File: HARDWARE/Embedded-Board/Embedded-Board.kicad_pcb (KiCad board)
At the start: 2 copper layers, 80 x 60 mm, 81 parts, among them J1 AD7265X, J11 USB_C_Receptacle_USB2.0, J2 POWER-pins, J3 Conn_02x20_Odd_Even, J4 AD7341, J5 I2C comm, J6 GPIO PINS, Q1 MMUN2133LT1G, SW1 SW_Push, SW2 RotaryEncoder_Switch, SW3 SW_Push_SPDT, SW5 BOOT, U1 MCP73831-2-OT, U18 LM1117-3.3, U2 W25Q16JVS, U3 RP2040, U4 TPS61090, Y1 12MHz

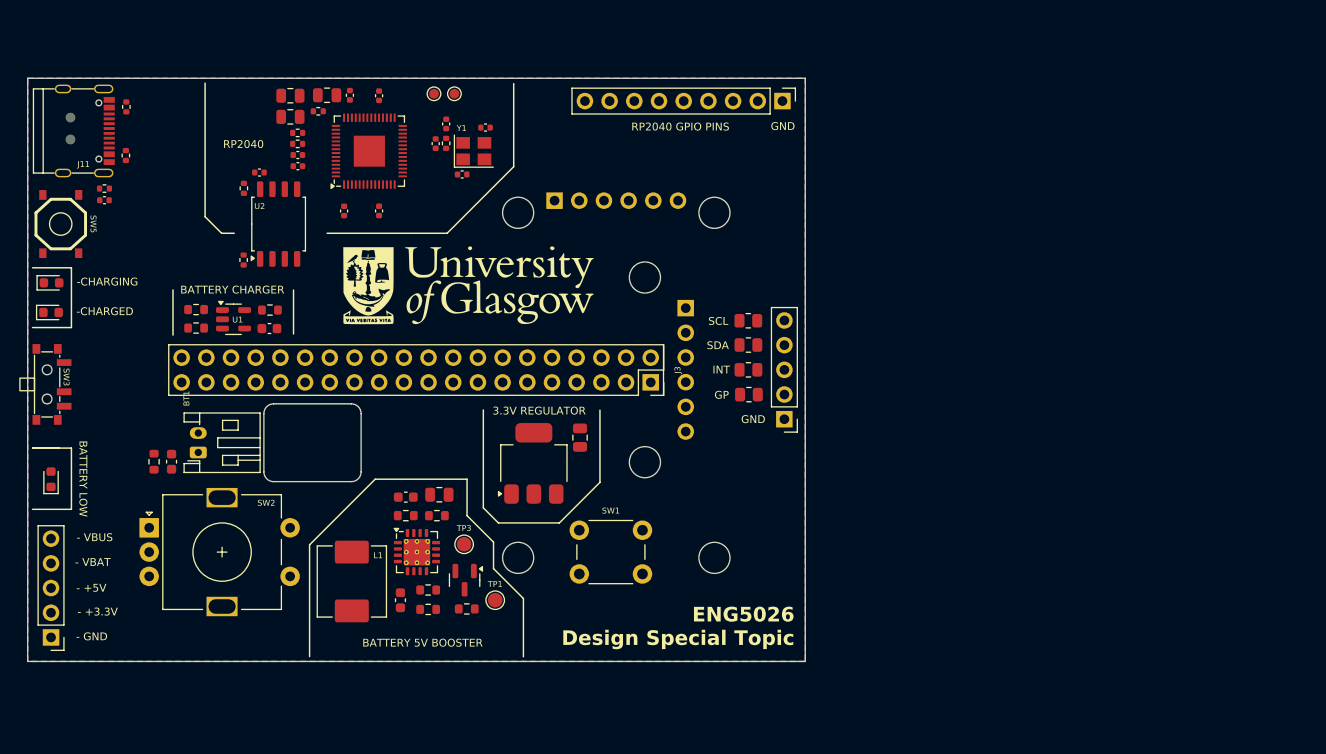
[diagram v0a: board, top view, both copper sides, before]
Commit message: Final PCB version
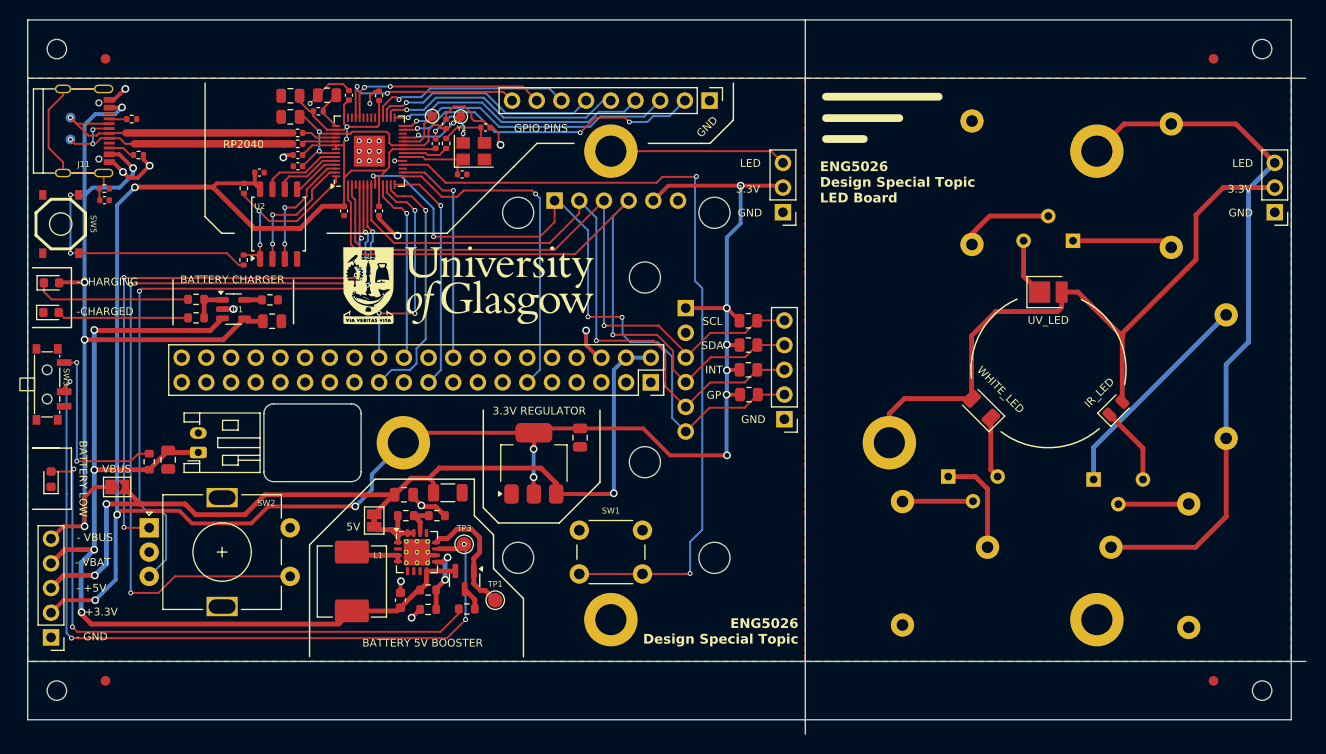
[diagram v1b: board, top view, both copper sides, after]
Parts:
- added D4: WHITE-LED, LED_SMD:LED_1206_3216Metric, F.Cu at (173.2, 88.6)
- added D5: IR_LED, LED_SMD:LED_0805_2012Metric, F.Cu at (187.1, 88.6)
- added D6: UV_LED, LED_SMD:LED_PLCC_2835, F.Cu at (180.2, 76.7)
- added G***: LOGO, test:uofg-8mm, B.Cu at (180.2, 84.7)
- added J7: BOARD->LED, Connector_PinHeader_2.54mm:PinHeader_1x03_P2.54mm_Vertical, F.Cu at (152.8, 68.4)
- added J8: LED->BOARD, Connector_PinHeader_2.54mm:PinHeader_1x03_P2.54mm_Vertical, F.Cu at (203.4, 68.4)
- added JP1: VBUS-5V, Jumper:SolderJumper-2_P1.3mm_Open_TrianglePad1.0x1.5mm, F.Cu at (84.3, 96.7)
- added JP2: OUT-5V, Jumper:SolderJumper-2_P1.3mm_Bridged_Pad1.0x1.5mm, F.Cu at (110.8, 100.2)
- added Q3: Q_NPN_BEC, Package_TO_SOT_THT:TO-92_Wide, B.Cu at (169.9, 95.6)
- added Q4: Q_NPN_BEC, Package_TO_SOT_THT:TO-92_Wide, B.Cu at (184.8, 95.9)
- added Q5: Q_NPN_BEC, Package_TO_SOT_THT:TO-92_Wide, B.Cu at (182.7, 71.4)
- added R23: 10k, Resistor_THT:R_Axial_DIN0411_L9.9mm_D3.6mm_P12.70mm_Horizontal, B.Cu at (186.6, 102.9)
- added R24: 10k, Resistor_THT:R_Axial_DIN0411_L9.9mm_D3.6mm_P12.70mm_Horizontal, B.Cu at (198.4, 91.7)
- added R25: 10k, Resistor_THT:R_Axial_DIN0411_L9.9mm_D3.6mm_P12.70mm_Horizontal, B.Cu at (192.8, 59.4)
- added R26: 470, Resistor_THT:R_Axial_DIN0411_L9.9mm_D3.6mm_P12.70mm_Horizontal, B.Cu at (165.2, 110.9)
- added R27: 470, Resistor_THT:R_Axial_DIN0411_L9.9mm_D3.6mm_P12.70mm_Horizontal, B.Cu at (194.6, 111.2)
- added R28: 470, Resistor_THT:R_Axial_DIN0411_L9.9mm_D3.6mm_P12.70mm_Horizontal, B.Cu at (172.3, 59.0)
- added REF**: Fiducial_1mm_Mask3mm, Fiducial:Fiducial_1mm_Mask3mm, F.Cu at (197.1, 116.6)
- added REF**: TestPoint, user:1.3mm_Test_Point, F.Cu at (202.2, 51.6)
- added REF**: Fiducial_1mm_Mask3mm, Fiducial:Fiducial_1mm_Mask3mm, F.Cu at (83.2, 52.7)
- added REF**: MountingHole_3.2mm_M3_ISO14580_Pad, MountingHole:MountingHole_3.2mm_M3_ISO14580_Pad, F.Cu at (185.2, 62.1)
- added REF**: TestPoint, user:1.3mm_Test_Point, F.Cu at (202.1, 117.7)
- added REF**: MountingHole_3.2mm_M3_ISO14580_Pad, MountingHole:MountingHole_3.2mm_M3_ISO14580_Pad, F.Cu at (135.2, 62.1)
- added REF**: MountingHole_3.2mm_M3_ISO14580_Pad, MountingHole:MountingHole_3.2mm_M3_ISO14580_Pad, F.Cu at (163.8, 92.2)
- added REF**: TestPoint, user:1.3mm_Test_Point, F.Cu at (78.2, 51.6)
- added REF**: Fiducial_1mm_Mask3mm, Fiducial:Fiducial_1mm_Mask3mm, F.Cu at (197.1, 52.7)
- added REF**: MountingHole_3.2mm_M3_ISO14580_Pad, MountingHole:MountingHole_3.2mm_M3_ISO14580_Pad, F.Cu at (185.2, 110.3)
- added REF**: MountingHole_3.2mm_M3_ISO14580_Pad, MountingHole:MountingHole_3.2mm_M3_ISO14580_Pad, F.Cu at (113.8, 92.2)
- added REF**: TestPoint, user:1.3mm_Test_Point, F.Cu at (78.2, 117.7)
- added REF**: Fiducial_1mm_Mask3mm, Fiducial:Fiducial_1mm_Mask3mm, F.Cu at (83.2, 116.6)
- added REF**: MountingHole_3.2mm_M3_ISO14580_Pad, MountingHole:MountingHole_3.2mm_M3_ISO14580_Pad, F.Cu at (135.2, 110.3)
- C2, C3, C5: footprint Capacitor_SMD:C_0603_1608Metric -> Capacitor_SMD:C_0805_2012Metric
- C6: footprint Capacitor_SMD:C_0805_2012Metric -> Capacitor_SMD:C_1206_3216Metric
- moved J6 7.50 mm to (145.3, 57.0)
- moved TP7 2.44 mm to (119.7, 58.6)
- moved TP6 2.31 mm to (116.8, 58.5)
- moved R13 1.37 mm to (85.8, 58.9), turned to 0 degrees
- moved R14 1.30 mm to (86.5, 62.5), turned to 180 degrees
- moved R6 1.05 mm to (92.5, 77.4)
- moved R8 1.05 mm to (92.5, 79.3)
- moved R9 1.05 mm to (100.1, 77.5)
- moved U1 1.05 mm to (96.3, 78.4)
- moved C6 0.90 mm to (118.4, 97.3)
- moved C2 0.80 mm to (100.3, 79.7)
- moved R17 0.50 mm to (87.7, 94.1)
- moved C3 0.40 mm to (89.6, 93.9)
- moved C5 0.32 mm to (113.8, 97.5)
- moved C19 0.10 mm to (108.2, 56.4)
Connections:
- R18 pad 2: +5V -> Net-(JP2-A)
- U3 pad 36: SENSOR-INT -> unconnected-(U3-GPIO24-Pad36)
- U3 pad 37: SENSOR-RST -> unconnected-(U3-GPIO25-Pad37)
- U3 pad 8: unconnected-(U3-GPIO6-Pad8) -> SENSOR-INT
- U3 pad 9: unconnected-(U3-GPIO7-Pad9) -> SENSOR-RST
- U4 pad 1: +5V -> Net-(JP2-A)
- U4 pad 15: +5V -> Net-(JP2-A)
- U4 pad 16: +5V -> Net-(JP2-A)
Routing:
- net +3.3V: track 0.00 -> 323.8 mm, vias 0 -> 14
- net +VBAT: track 0.00 -> 102.3 mm, vias 0 -> 4
- net +5V: track 0.00 -> 93.5 mm, vias 0 -> 3
- net LED-BOARD: track 0.00 -> 90.9 mm
- net VBUS: track 0.00 -> 88.9 mm, vias 0 -> 5
- net PUSH-SWITCH: track 0.00 -> 84.4 mm, vias 0 -> 2
- net ENC-PSH: track 0.00 -> 83.1 mm, vias 0 -> 4
- net Net-(SW3-B): track 0.00 -> 80.0 mm, vias 0 -> 4
- net SENSOR-SDA: track 0.00 -> 74.4 mm, vias 0 -> 1
- net SENSOR-RST: track 0.00 -> 71.7 mm, vias 0 -> 4
- net SENSOR-INT: track 0.00 -> 69.5 mm, vias 0 -> 1
- net SENSOR-SCL: track 0.00 -> 68.7 mm, vias 0 -> 1
- net ENC-B: track 0.00 -> 66.6 mm, vias 0 -> 3
- net ENC-A: track 0.00 -> 62.0 mm, vias 0 -> 4
- net Net-(D3-A): track 0.00 -> 60.0 mm, vias 0 -> 2
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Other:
- board size 80 x 60 mm -> 131.5 x 73.5 mm
- board text added: "3.3V"
- board text added: "5V"
- board text added: "CNC"
- board text added: "Drawn by Nicolas Viale"
- board text added: "ENG5026 Design Special Topic LED Board"
- board text added: "GPIO PINS"
- board text added: "IR_LED"
- board text added: "LED"
- board text added: "Schematic & PCB"
- board text added: "Spectrometer Board LED board v1.0 Apr. 2025"
- board text added: "Spectrometer Board v1.0 Apr. 2025"
- board text added: "UV_LED"
- board text added: "V-CUT"
- board text added: "VBUS"
- board text added: "WHITE_LED"
- board text added: "~10k"
- board text added: "~470"
- board text removed: "RP2040 GPIO PINS"
- board text removed: "Schematic & PCB drawn by Nicolas Viale"
